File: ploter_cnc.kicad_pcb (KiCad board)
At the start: 2 copper layers, 90 x 60 mm, 13 parts, among them J1 Conn_01x05_Socket, J2 Conn_01x05_Socket, J3 Conn_01x05_Socket, J4 Conn_01x02_Socket, U1 ULN2803A, U2 ULN2803A

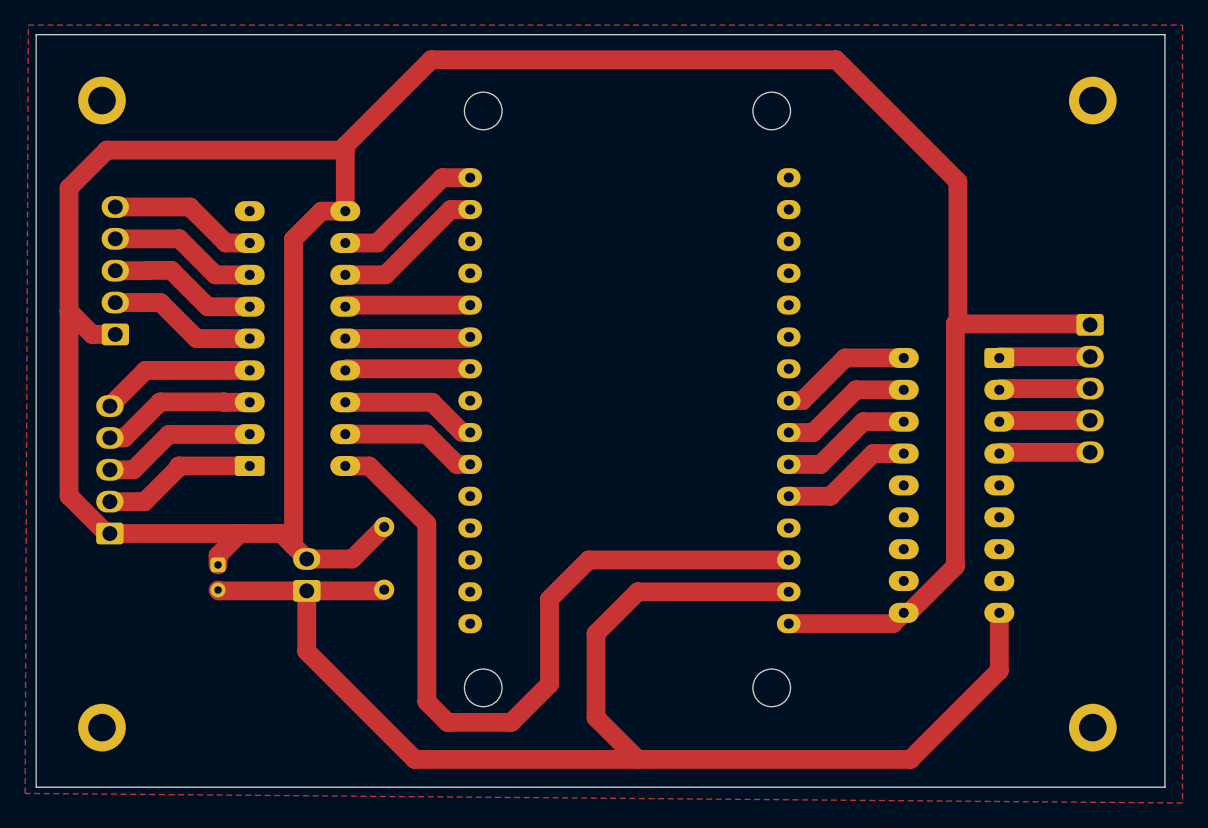
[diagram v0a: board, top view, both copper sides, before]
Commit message: xlas
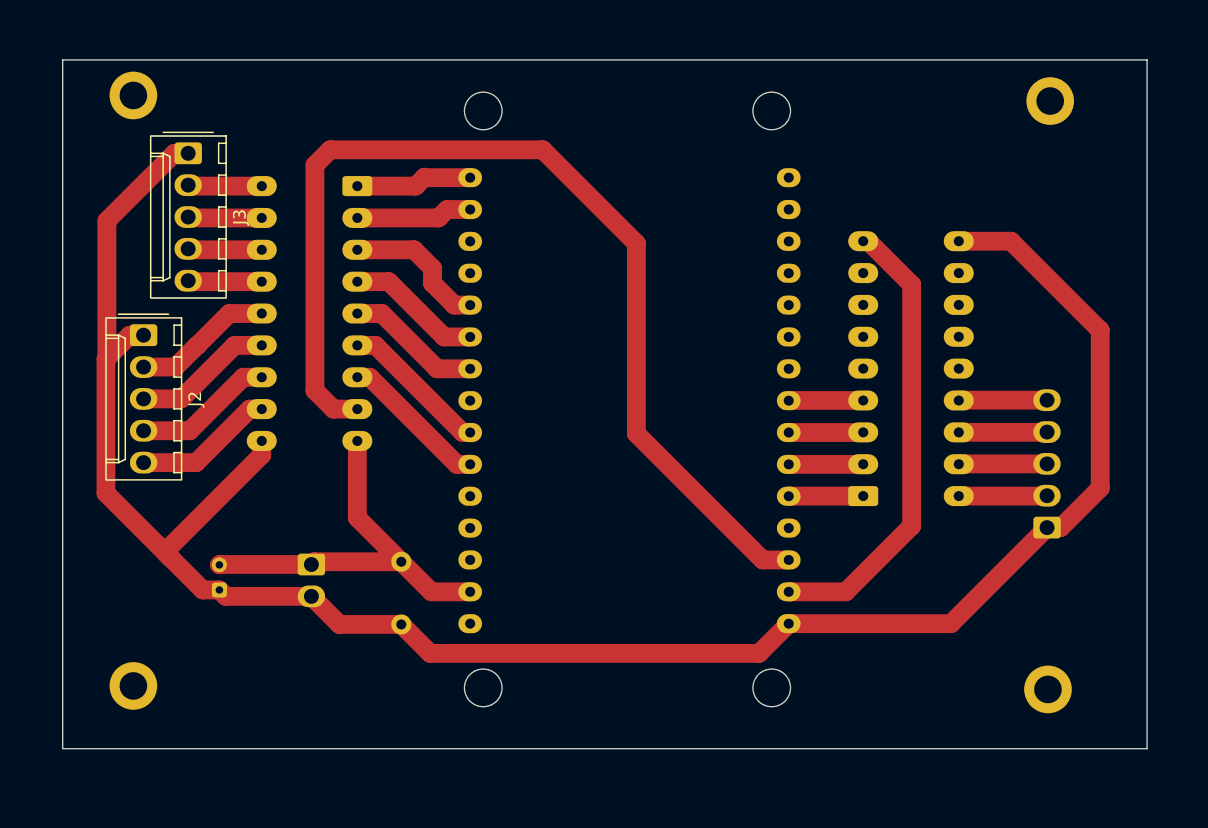
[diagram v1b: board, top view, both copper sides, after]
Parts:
- J2, J3: moved to F.Cu
- moved U2 23.9 mm to (132.8, 84.1), turned to 180 degrees
- moved J1 16.5 mm to (187.8, 111.3), turned to 90 degrees
- moved J2 16.0 mm to (115.8, 96.0), turned to -90 degrees
- moved J3 15.6 mm to (119.4, 81.5), turned to -90 degrees
- moved U1 15.5 mm to (173.2, 108.8), turned to 0 degrees
- moved C1 7.89 mm to (136.3, 119.0), turned to 90 degrees
- moved H2 4.70 mm to (187.9, 124.2)
- moved H3 4.16 mm to (115.0, 123.9)
- moved H1 3.40 mm to (188.1, 77.3)
- moved H4 2.53 mm to (115.0, 76.8)
- moved J4 2.13 mm to (129.2, 114.2), turned to -90 degrees
- moved C2 2.00 mm to (121.8, 116.3), turned to 90 degrees
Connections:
- J2 pad 2: A1 -> Net-(J2-Pin_2)
- J2 pad 3: B1 -> Net-(J2-Pin_3)
- J2 pad 4: C1 -> Net-(J2-Pin_4)
- J2 pad 5: D1 -> Net-(J2-Pin_5)
- J3 pad 2: A2 -> D2
- J3 pad 3: B2 -> C2
- J3 pad 4: C2 -> B2
- J3 pad 5: D2 -> A2
- U1 pad 1: A -> Net-(U1-I1)
- U1 pad 15: Net-(U1-O4) -> D
- U1 pad 16: Net-(U1-O3) -> C
- U1 pad 17: Net-(U1-O2) -> B
- U1 pad 18: Net-(U1-O1) -> A
- U1 pad 2: B -> Net-(U1-I2)
- U1 pad 3: C -> Net-(U1-I3)
- U1 pad 4: D -> Net-(U1-I4)
- U2 pad 1: A1 -> Net-(U2-I1)
- U2 pad 11: Net-(U2-O8) -> Net-(J2-Pin_5)
- U2 pad 12: Net-(U2-O7) -> Net-(J2-Pin_4)
- U2 pad 13: Net-(U2-O6) -> Net-(J2-Pin_3)
- U2 pad 14: Net-(U2-O5) -> Net-(J2-Pin_2)
- U2 pad 15: Net-(U2-O4) -> A2
- U2 pad 16: Net-(U2-O3) -> B2
- U2 pad 17: Net-(U2-O2) -> C2
- U2 pad 18: Net-(U2-O1) -> D2
- U2 pad 2: B1 -> Net-(U2-I2)
- U2 pad 3: C1 -> Net-(U2-I3)
- U2 pad 4: D1 -> Net-(U2-I4)
- U2 pad 5: A2 -> Net-(U2-I5)
- U2 pad 6: B2 -> Net-(U2-I6)
- U2 pad 7: C2 -> Net-(U2-I7)
- U2 pad 8: D2 -> Net-(U2-I8)
- U3 pad 21: Net-(U2-O2) -> Net-(U2-I7)
- U3 pad 22: Net-(U2-O3) -> Net-(U2-I6)
- U3 pad 24: Net-(U2-O4) -> Net-(U2-I5)
- U3 pad 25: Net-(U2-O5) -> Net-(U2-I4)
- U3 pad 26: Net-(U2-O6) -> Net-(U2-I3)
- U3 pad 29: Net-(U2-O7) -> Net-(U2-I2)
- U3 pad 3: Net-(U2-O1) -> Net-(U2-I8)
- U3 pad 30: Net-(U2-O8) -> Net-(U2-I1)
- U3 pad 5: Net-(U1-O4) -> Net-(U1-I1)
- U3 pad 6: Net-(U1-O3) -> Net-(U1-I2)
- U3 pad 7: Net-(U1-O2) -> Net-(U1-I3)
- U3 pad 8: Net-(U1-O1) -> Net-(U1-I4)
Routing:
- net Net-(U2-I8): track 0.00 -> 82.7 mm
- net VCC: track 230.9 -> 164.5 mm
- net Net-(U2-O1): track 61.5 -> 0.00 mm
- net GND: track 112.6 -> 68.7 mm
- net A1: track 12.4 -> 0.00 mm
- net C1: track 12.3 -> 0.00 mm
- net B1: track 12.3 -> 0.00 mm
- net D1: track 12.3 -> 0.00 mm
- net Net-(U2-O7): track 12.1 -> 0.00 mm
- net Net-(U2-O8): track 12.1 -> 0.00 mm
- net Net-(U2-I7): track 0.00 -> 11.9 mm
- net Net-(U2-I6): track 0.00 -> 11.9 mm
- net Net-(U2-I3): track 0.00 -> 11.5 mm
- net Net-(J2-Pin_5): track 0.00 -> 11.2 mm
- net Net-(J2-Pin_4): track 0.00 -> 11.2 mm
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- removed copper zone on F.Cu, net GND
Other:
- board size 90 x 60 mm -> 86.5 x 54.9 mm
